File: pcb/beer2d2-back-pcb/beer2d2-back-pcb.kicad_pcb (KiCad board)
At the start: 2 copper layers, 233 parts, among them IC1 74HC238, IC2 TLC5971, IC3 FT230X, IC4 LM1117, IC5 ATMEGA328P, J1 USB, J2 PSI1, J3 PSI2, J4 RGB1, J5 RGB2, J6 6-12V, P1 AVR_ISP, Q1 DDTD113ZC, Q10 DDTB113ZC, Q11 DDTB113ZC, Q12 DDTB113ZC, Q13 DDTB113ZC, Q14 DDTB113ZC, Q15 DDTB113ZC, Q16 DDTB113ZC, Q17 DDTB113ZC, Q18 DDTB113ZC, Q19 DDTB113ZC, Q2 DDTD113ZC, Q3 DDTD113ZC, Q4 DDTD113ZC, Q5 DDTD113ZC, Q6 DDTD113ZC, Q7 DDTD113ZC, Q8 DDTD113ZC, Q9 DDTB113ZC, Y1 16MHz

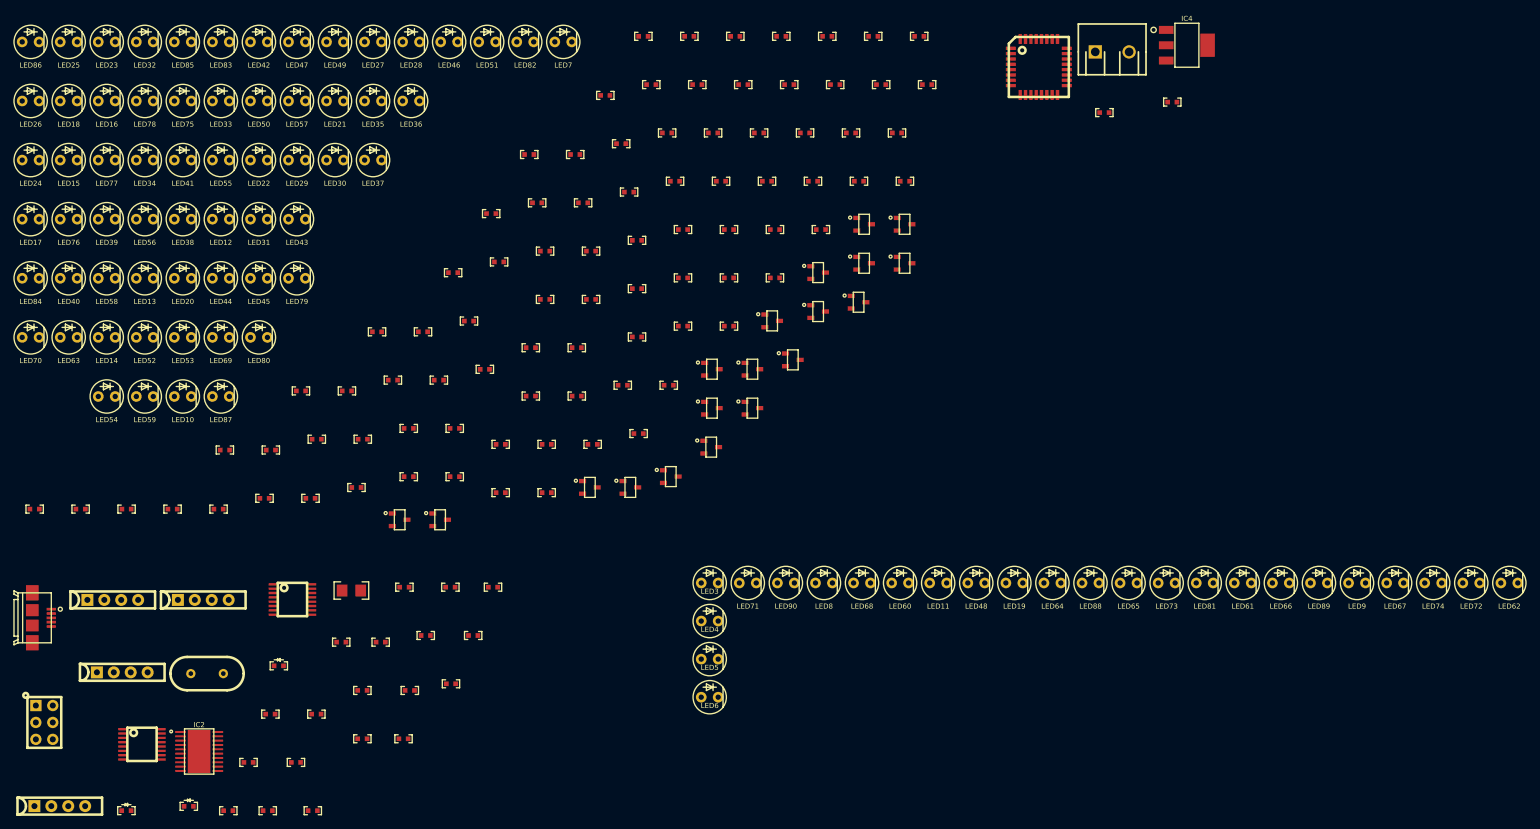
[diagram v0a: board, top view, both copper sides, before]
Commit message: tentative placement layout
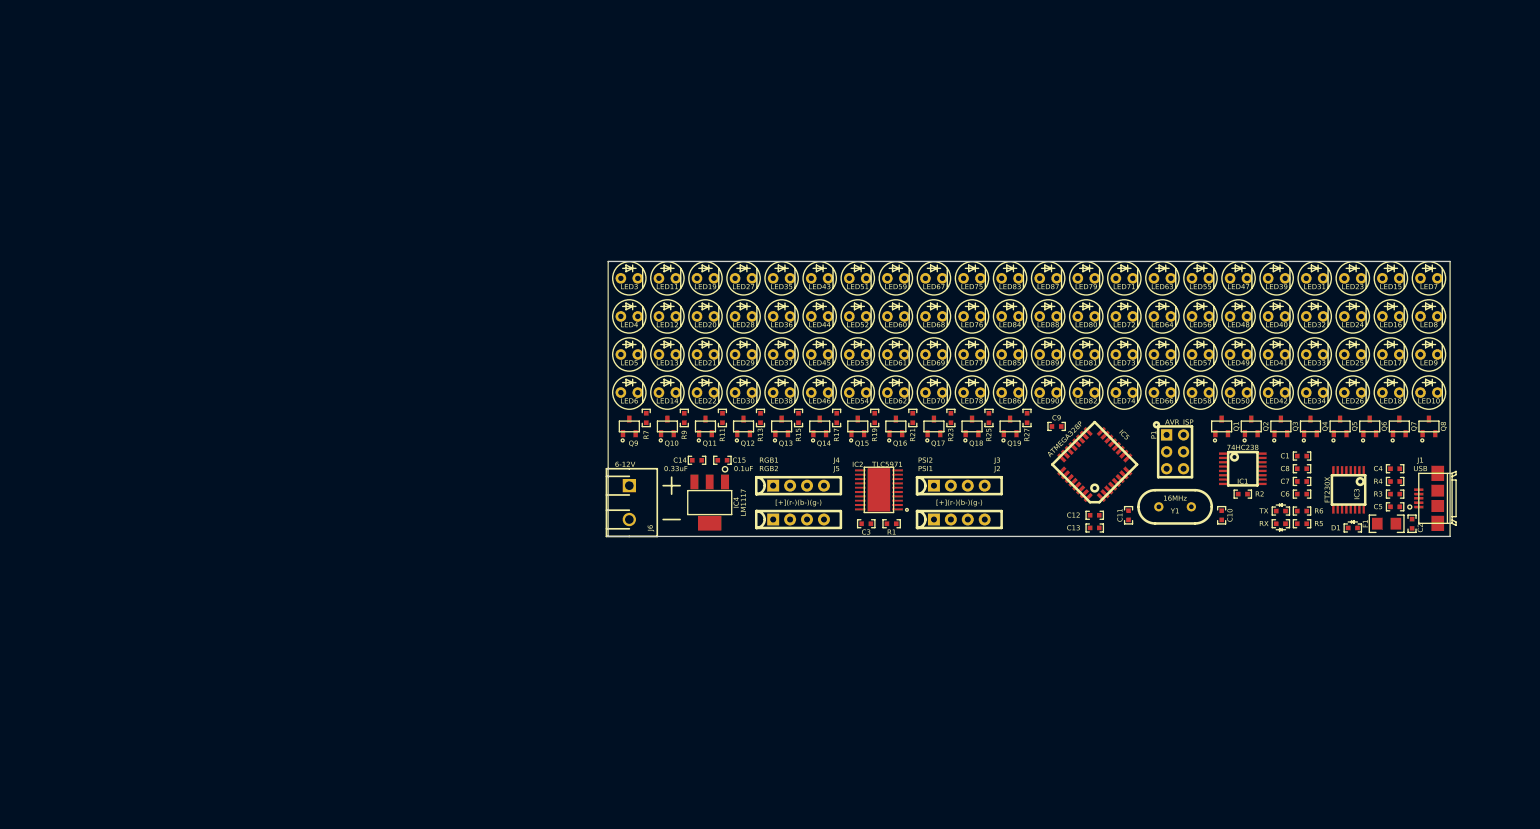
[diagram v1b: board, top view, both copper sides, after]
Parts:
- removed R10, R12, R14, R16, R18, R20, R22, R24, R26, R28, R29, R30, R31, R32, R33, R34, R35, R36, R37, R38, R39, R40, R41, R42, R43, R44, R45, R46, R47, R48, R49, R50, R51, R52, R53, R54, R55, R56, R57, R58, R59, R60, R61, R62, R63, R64, R65, R66, R67, R68, R69, R70, R71, R72, R73, R74, R75, R76, R77, R78, R79, R8, R80, R81, R82, R83, R84, R85, R86, R87, R88, R89, R90, R91, R92, R93, R94: 110Ω, general sm:0603(1608m)
- moved J1 211.6 mm to (257.2, 112.4), turned to 180 degrees
- moved LED17 205.2 mm to (250.2, 90.8)
- moved LED18 203.2 mm to (250.2, 96.5)
- moved LED26 203.2 mm to (244.5, 96.5)
- moved LED24 199.8 mm to (244.5, 85.1)
- moved LED15 199.2 mm to (250.2, 79.4)
- moved LED25 198.4 mm to (244.5, 90.8)
- moved LED16 195.4 mm to (250.2, 85.1)
- moved LED23 190.4 mm to (244.5, 79.4)
- moved LED10 187.0 mm to (255.9, 96.5)
- moved IC3 185.1 mm to (243.8, 111.1), turned to 270 degrees
- moved R3 181.5 mm to (250.8, 111.8), turned to 180 degrees
- moved LED40 181.4 mm to (233.0, 85.1)
- moved LED32 180.4 mm to (238.8, 85.1)
- moved LED34 179.0 mm to (238.8, 96.5)
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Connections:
- IC2 pad 11: Net-(IC2-Pad11) -> (no net)
- IC2 pad 12: Net-(IC2-Pad12) -> (no net)
- IC3 pad 15: Net-(IC3-Pad15) -> (no net)
- IC3 pad 6: Net-(IC3-Pad6) -> (no net)
- IC5 pad 19: Net-(IC5-Pad19) -> (no net)
- IC5 pad 22: Net-(IC5-Pad22) -> (no net)
- IC5 pad 26: Net-(IC5-Pad26) -> (no net)
- J1 pad 4: Net-(J1-Pad4) -> (no net)
- LED10 pad 1: Net-(LED10-Pad1) -> /LED Matrix/ROW7
- LED10 pad 2: /LED Matrix/COL0 -> N-0000097
- LED11 pad 1: Net-(LED11-Pad1) -> /LED Matrix/ROW0
- LED11 pad 2: /LED Matrix/COL1 -> N-0000096
- LED12 pad 1: Net-(LED12-Pad1) -> /LED Matrix/ROW1
- LED12 pad 2: /LED Matrix/COL1 -> N-0000096
- LED13 pad 1: Net-(LED13-Pad1) -> /LED Matrix/ROW2
- LED13 pad 2: /LED Matrix/COL1 -> N-0000096
- LED14 pad 1: Net-(LED14-Pad1) -> /LED Matrix/ROW3
- LED14 pad 2: /LED Matrix/COL1 -> N-0000096
- LED15 pad 1: Net-(LED15-Pad1) -> /LED Matrix/ROW4
- LED15 pad 2: /LED Matrix/COL1 -> N-0000096
- LED16 pad 1: Net-(LED16-Pad1) -> /LED Matrix/ROW5
- LED16 pad 2: /LED Matrix/COL1 -> N-0000096
- LED17 pad 1: Net-(LED17-Pad1) -> /LED Matrix/ROW6
- LED17 pad 2: /LED Matrix/COL1 -> N-0000096
- LED18 pad 1: Net-(LED18-Pad1) -> /LED Matrix/ROW7
- LED18 pad 2: /LED Matrix/COL1 -> N-0000096
- LED19 pad 1: Net-(LED19-Pad1) -> /LED Matrix/ROW0
- LED19 pad 2: /LED Matrix/COL2 -> N-0000098
- LED20 pad 1: Net-(LED20-Pad1) -> /LED Matrix/ROW1
- LED20 pad 2: /LED Matrix/COL2 -> N-0000098
- LED21 pad 1: Net-(LED21-Pad1) -> /LED Matrix/ROW2
- LED21 pad 2: /LED Matrix/COL2 -> N-0000098
- LED22 pad 1: Net-(LED22-Pad1) -> /LED Matrix/ROW3
- LED22 pad 2: /LED Matrix/COL2 -> N-0000098
- LED23 pad 1: Net-(LED23-Pad1) -> /LED Matrix/ROW4
- LED23 pad 2: /LED Matrix/COL2 -> N-0000098
- LED24 pad 1: Net-(LED24-Pad1) -> /LED Matrix/ROW5
- LED24 pad 2: /LED Matrix/COL2 -> N-0000098
- LED25 pad 1: Net-(LED25-Pad1) -> /LED Matrix/ROW6
- LED25 pad 2: /LED Matrix/COL2 -> N-0000098
- LED26 pad 1: Net-(LED26-Pad1) -> /LED Matrix/ROW7
- LED26 pad 2: /LED Matrix/COL2 -> N-0000098
- LED27 pad 1: Net-(LED27-Pad1) -> /LED Matrix/ROW0
- LED27 pad 2: /LED Matrix/COL3 -> N-0000094
- LED28 pad 1: Net-(LED28-Pad1) -> /LED Matrix/ROW1
- LED28 pad 2: /LED Matrix/COL3 -> N-0000094
- LED29 pad 1: Net-(LED29-Pad1) -> /LED Matrix/ROW2
- LED29 pad 2: /LED Matrix/COL3 -> N-0000094
- LED3 pad 1: Net-(LED3-Pad1) -> /LED Matrix/ROW0
- LED3 pad 2: /LED Matrix/COL0 -> N-0000097
- LED30 pad 1: Net-(LED30-Pad1) -> /LED Matrix/ROW3
- LED30 pad 2: /LED Matrix/COL3 -> N-0000094
- LED31 pad 1: Net-(LED31-Pad1) -> /LED Matrix/ROW4
- LED31 pad 2: /LED Matrix/COL3 -> N-0000094
- LED32 pad 1: Net-(LED32-Pad1) -> /LED Matrix/ROW5
- LED32 pad 2: /LED Matrix/COL3 -> N-0000094
- LED33 pad 1: Net-(LED33-Pad1) -> /LED Matrix/ROW6
- LED33 pad 2: /LED Matrix/COL3 -> N-0000094
- LED34 pad 1: Net-(LED34-Pad1) -> /LED Matrix/ROW7
- LED34 pad 2: /LED Matrix/COL3 -> N-0000094
- LED35 pad 1: Net-(LED35-Pad1) -> /LED Matrix/ROW0
- LED35 pad 2: /LED Matrix/COL4 -> N-0000093
- LED36 pad 1: Net-(LED36-Pad1) -> /LED Matrix/ROW1
- LED36 pad 2: /LED Matrix/COL4 -> N-0000093
- LED37 pad 1: Net-(LED37-Pad1) -> /LED Matrix/ROW2
- LED37 pad 2: /LED Matrix/COL4 -> N-0000093
- LED38 pad 1: Net-(LED38-Pad1) -> /LED Matrix/ROW3
- LED38 pad 2: /LED Matrix/COL4 -> N-0000093
- LED39 pad 1: Net-(LED39-Pad1) -> /LED Matrix/ROW4
- LED39 pad 2: /LED Matrix/COL4 -> N-0000093
- LED4 pad 1: Net-(LED4-Pad1) -> /LED Matrix/ROW1
- LED4 pad 2: /LED Matrix/COL0 -> N-0000097
- LED40 pad 1: Net-(LED40-Pad1) -> /LED Matrix/ROW5
- LED40 pad 2: /LED Matrix/COL4 -> N-0000093
- LED41 pad 1: Net-(LED41-Pad1) -> /LED Matrix/ROW6
- LED41 pad 2: /LED Matrix/COL4 -> N-0000093
- LED42 pad 1: Net-(LED42-Pad1) -> /LED Matrix/ROW7
- LED42 pad 2: /LED Matrix/COL4 -> N-0000093
- LED43 pad 1: Net-(LED43-Pad1) -> /LED Matrix/ROW0
- LED43 pad 2: /LED Matrix/COL5 -> N-0000095
- LED44 pad 1: Net-(LED44-Pad1) -> /LED Matrix/ROW1
- LED44 pad 2: /LED Matrix/COL5 -> N-0000095
- LED45 pad 1: Net-(LED45-Pad1) -> /LED Matrix/ROW2
- LED45 pad 2: /LED Matrix/COL5 -> N-0000095
- LED46 pad 1: Net-(LED46-Pad1) -> /LED Matrix/ROW3
- LED46 pad 2: /LED Matrix/COL5 -> N-0000095
- LED47 pad 1: Net-(LED47-Pad1) -> /LED Matrix/ROW4
- LED47 pad 2: /LED Matrix/COL5 -> N-0000095
- LED48 pad 1: Net-(LED48-Pad1) -> /LED Matrix/ROW5
- LED48 pad 2: /LED Matrix/COL5 -> N-0000095
- LED49 pad 1: Net-(LED49-Pad1) -> /LED Matrix/ROW6
- LED49 pad 2: /LED Matrix/COL5 -> N-0000095
- LED5 pad 1: Net-(LED5-Pad1) -> /LED Matrix/ROW2
- LED5 pad 2: /LED Matrix/COL0 -> N-0000097
- LED50 pad 1: Net-(LED50-Pad1) -> /LED Matrix/ROW7
- LED50 pad 2: /LED Matrix/COL5 -> N-0000095
- LED51 pad 1: Net-(LED51-Pad1) -> /LED Matrix/ROW0
- LED51 pad 2: /LED Matrix/COL6 -> N-0000081
- LED52 pad 1: Net-(LED52-Pad1) -> /LED Matrix/ROW1
- LED52 pad 2: /LED Matrix/COL6 -> N-0000081
- LED53 pad 1: Net-(LED53-Pad1) -> /LED Matrix/ROW2
- LED53 pad 2: /LED Matrix/COL6 -> N-0000081
- LED54 pad 1: Net-(LED54-Pad1) -> /LED Matrix/ROW3
- LED54 pad 2: /LED Matrix/COL6 -> N-0000081
- LED55 pad 1: Net-(LED55-Pad1) -> /LED Matrix/ROW4
- LED55 pad 2: /LED Matrix/COL6 -> N-0000081
- LED56 pad 1: Net-(LED56-Pad1) -> /LED Matrix/ROW5
- LED56 pad 2: /LED Matrix/COL6 -> N-0000081
- LED57 pad 1: Net-(LED57-Pad1) -> /LED Matrix/ROW6
- LED57 pad 2: /LED Matrix/COL6 -> N-0000081
- LED58 pad 1: Net-(LED58-Pad1) -> /LED Matrix/ROW7
- LED58 pad 2: /LED Matrix/COL6 -> N-0000081
- LED59 pad 1: Net-(LED59-Pad1) -> /LED Matrix/ROW0
- LED59 pad 2: /LED Matrix/COL7 -> N-0000082
- LED6 pad 1: Net-(LED6-Pad1) -> /LED Matrix/ROW3
- LED6 pad 2: /LED Matrix/COL0 -> N-0000097
- LED60 pad 1: Net-(LED60-Pad1) -> /LED Matrix/ROW1
- LED60 pad 2: /LED Matrix/COL7 -> N-0000082
- LED61 pad 1: Net-(LED61-Pad1) -> /LED Matrix/ROW2
- LED61 pad 2: /LED Matrix/COL7 -> N-0000082
- LED62 pad 1: Net-(LED62-Pad1) -> /LED Matrix/ROW3
- LED62 pad 2: /LED Matrix/COL7 -> N-0000082
- LED63 pad 1: Net-(LED63-Pad1) -> /LED Matrix/ROW4
- LED63 pad 2: /LED Matrix/COL7 -> N-0000082
- LED64 pad 1: Net-(LED64-Pad1) -> /LED Matrix/ROW5
- LED64 pad 2: /LED Matrix/COL7 -> N-0000082
- LED65 pad 1: Net-(LED65-Pad1) -> /LED Matrix/ROW6
- LED65 pad 2: /LED Matrix/COL7 -> N-0000082
- LED66 pad 1: Net-(LED66-Pad1) -> /LED Matrix/ROW7
- LED66 pad 2: /LED Matrix/COL7 -> N-0000082
- LED67 pad 1: Net-(LED67-Pad1) -> /LED Matrix/ROW0
- LED67 pad 2: /LED Matrix/COL8 -> N-0000080
- LED68 pad 1: Net-(LED68-Pad1) -> /LED Matrix/ROW1
- LED68 pad 2: /LED Matrix/COL8 -> N-0000080
- LED69 pad 1: Net-(LED69-Pad1) -> /LED Matrix/ROW2
- LED69 pad 2: /LED Matrix/COL8 -> N-0000080
- LED7 pad 1: Net-(LED7-Pad1) -> /LED Matrix/ROW4
- LED7 pad 2: /LED Matrix/COL0 -> N-0000097
- LED70 pad 1: Net-(LED70-Pad1) -> /LED Matrix/ROW3
- LED70 pad 2: /LED Matrix/COL8 -> N-0000080
- LED71 pad 1: Net-(LED71-Pad1) -> /LED Matrix/ROW4
- LED71 pad 2: /LED Matrix/COL8 -> N-0000080
- LED72 pad 1: Net-(LED72-Pad1) -> /LED Matrix/ROW5
- LED72 pad 2: /LED Matrix/COL8 -> N-0000080
- LED73 pad 1: Net-(LED73-Pad1) -> /LED Matrix/ROW6
- LED73 pad 2: /LED Matrix/COL8 -> N-0000080
- LED74 pad 1: Net-(LED74-Pad1) -> /LED Matrix/ROW7
- LED74 pad 2: /LED Matrix/COL8 -> N-0000080
- LED75 pad 1: Net-(LED75-Pad1) -> /LED Matrix/ROW0
- LED75 pad 2: /LED Matrix/COL9 -> N-0000085
- LED76 pad 1: Net-(LED76-Pad1) -> /LED Matrix/ROW1
- LED76 pad 2: /LED Matrix/COL9 -> N-0000085
- LED77 pad 1: Net-(LED77-Pad1) -> /LED Matrix/ROW2
- LED77 pad 2: /LED Matrix/COL9 -> N-0000085
- LED78 pad 1: Net-(LED78-Pad1) -> /LED Matrix/ROW3
- LED78 pad 2: /LED Matrix/COL9 -> N-0000085
- LED79 pad 1: Net-(LED79-Pad1) -> /LED Matrix/ROW4
- LED79 pad 2: /LED Matrix/COL9 -> N-0000085
- LED8 pad 1: Net-(LED8-Pad1) -> /LED Matrix/ROW5
- LED8 pad 2: /LED Matrix/COL0 -> N-0000097
- LED80 pad 1: Net-(LED80-Pad1) -> /LED Matrix/ROW5
- LED80 pad 2: /LED Matrix/COL9 -> N-0000085
- LED81 pad 1: Net-(LED81-Pad1) -> /LED Matrix/ROW6
- LED81 pad 2: /LED Matrix/COL9 -> N-0000085
- LED82 pad 1: Net-(LED82-Pad1) -> /LED Matrix/ROW7
- LED82 pad 2: /LED Matrix/COL9 -> N-0000085
- LED83 pad 1: Net-(LED83-Pad1) -> /LED Matrix/ROW0
- LED83 pad 2: /LED Matrix/COL10 -> N-0000074
- LED84 pad 1: Net-(LED84-Pad1) -> /LED Matrix/ROW1
- LED84 pad 2: /LED Matrix/COL10 -> N-0000074
- LED85 pad 1: Net-(LED85-Pad1) -> /LED Matrix/ROW2
- LED85 pad 2: /LED Matrix/COL10 -> N-0000074
- LED86 pad 1: Net-(LED86-Pad1) -> /LED Matrix/ROW3
- LED86 pad 2: /LED Matrix/COL10 -> N-0000074
- LED87 pad 1: Net-(LED87-Pad1) -> /LED Matrix/ROW4
- LED87 pad 2: /LED Matrix/COL10 -> N-0000074
- LED88 pad 1: Net-(LED88-Pad1) -> /LED Matrix/ROW5
- LED88 pad 2: /LED Matrix/COL10 -> N-0000074
- LED89 pad 1: Net-(LED89-Pad1) -> /LED Matrix/ROW6
- LED89 pad 2: /LED Matrix/COL10 -> N-0000074
- LED9 pad 1: Net-(LED9-Pad1) -> /LED Matrix/ROW6
- LED9 pad 2: /LED Matrix/COL0 -> N-0000097
- LED90 pad 1: Net-(LED90-Pad1) -> /LED Matrix/ROW7
- LED90 pad 2: /LED Matrix/COL10 -> N-0000074
- R11 pad 1: /LED Matrix/ROW4 -> /LED Matrix/COL2
- R11 pad 2: Net-(LED7-Pad1) -> N-0000098
- R13 pad 1: /LED Matrix/ROW6 -> /LED Matrix/COL3
- R13 pad 2: Net-(LED9-Pad1) -> N-0000094
- R15 pad 1: /LED Matrix/ROW0 -> /LED Matrix/COL4
- R15 pad 2: Net-(LED11-Pad1) -> N-0000093
- R17 pad 1: /LED Matrix/ROW2 -> /LED Matrix/COL5
- R17 pad 2: Net-(LED13-Pad1) -> N-0000095
- R19 pad 1: /LED Matrix/ROW4 -> /LED Matrix/COL6
- R19 pad 2: Net-(LED15-Pad1) -> N-0000081
- R21 pad 1: /LED Matrix/ROW6 -> /LED Matrix/COL7
- R21 pad 2: Net-(LED17-Pad1) -> N-0000082
- R23 pad 1: /LED Matrix/ROW0 -> /LED Matrix/COL8
- R23 pad 2: Net-(LED19-Pad1) -> N-0000080
- R25 pad 1: /LED Matrix/ROW2 -> /LED Matrix/COL9
- R25 pad 2: Net-(LED21-Pad1) -> N-0000085
- R27 pad 1: /LED Matrix/ROW4 -> /LED Matrix/COL10
- R27 pad 2: Net-(LED23-Pad1) -> N-0000074
- R7 pad 1: /LED Matrix/ROW0 -> /LED Matrix/COL0
- R7 pad 2: Net-(LED3-Pad1) -> N-0000097
- R9 pad 1: /LED Matrix/ROW2 -> /LED Matrix/COL1
- R9 pad 2: Net-(LED5-Pad1) -> N-0000096
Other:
- board outline added: 126.4 x 41.3 mm
- board text added: "[+](r-)(b-)(g-)"
